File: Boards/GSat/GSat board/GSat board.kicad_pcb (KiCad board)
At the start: 2 copper layers, 75 x 108 mm, 33 parts, among them IC2 MCP23017-E_SP, IC3 SP3485CN-L_TR, J1 B3B-XH-A_LF__SN_, J10 Conn_01x05_Pin, J11 Conn_01x06_Pin, J13 B4B-XH-A_LF__SN_, J14 B4B-XH-A_LF__SN_, J15 B4B-XH-A_LF__SN_, J16 B4B-XH-A_LF__SN_, J3 B3B-XH-A_LF__SN_, J4 B3B-XH-A_LF__SN_, J5 1723163304, U1 TMC2209_SILENTSTEPSTICK, U2 TMC2209_SILENTSTEPSTICK, U3 E28-2G4M27SX, U4 LD1117S33TR_SOT223

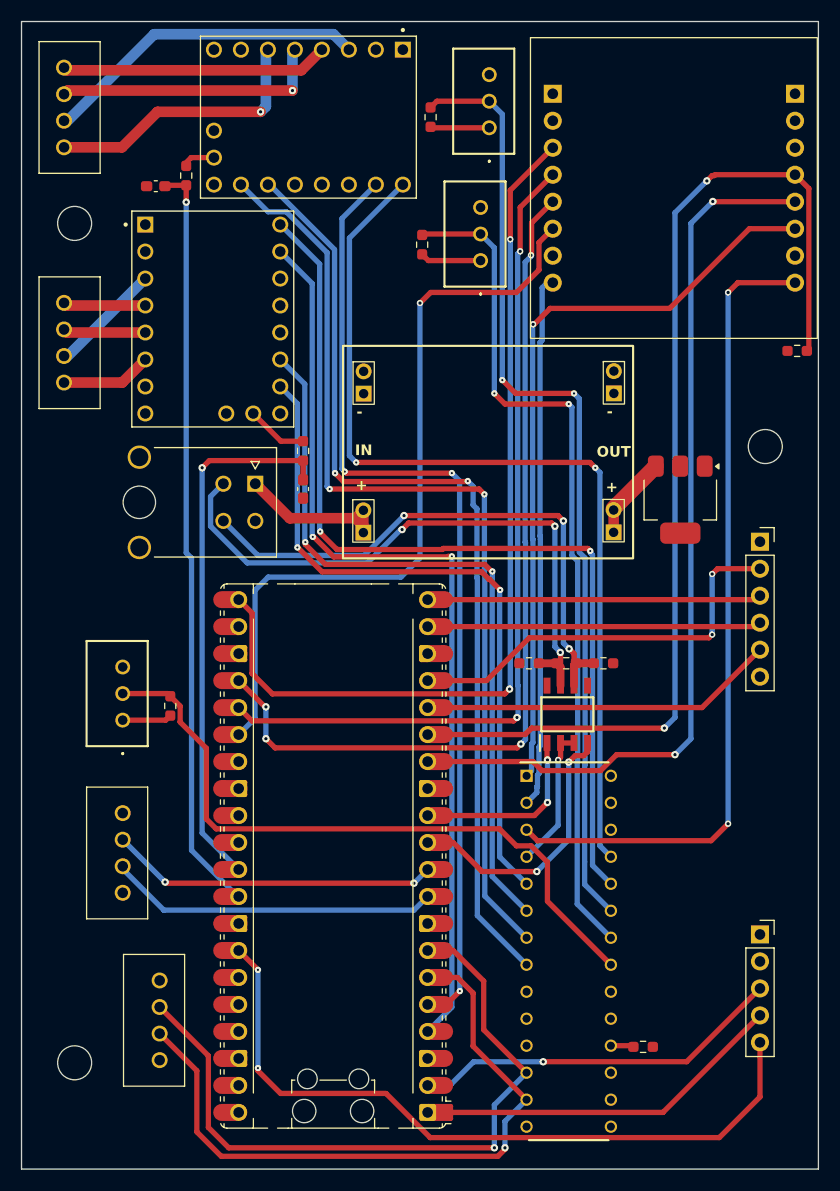
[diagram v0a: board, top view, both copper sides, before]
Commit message: GSPOT update
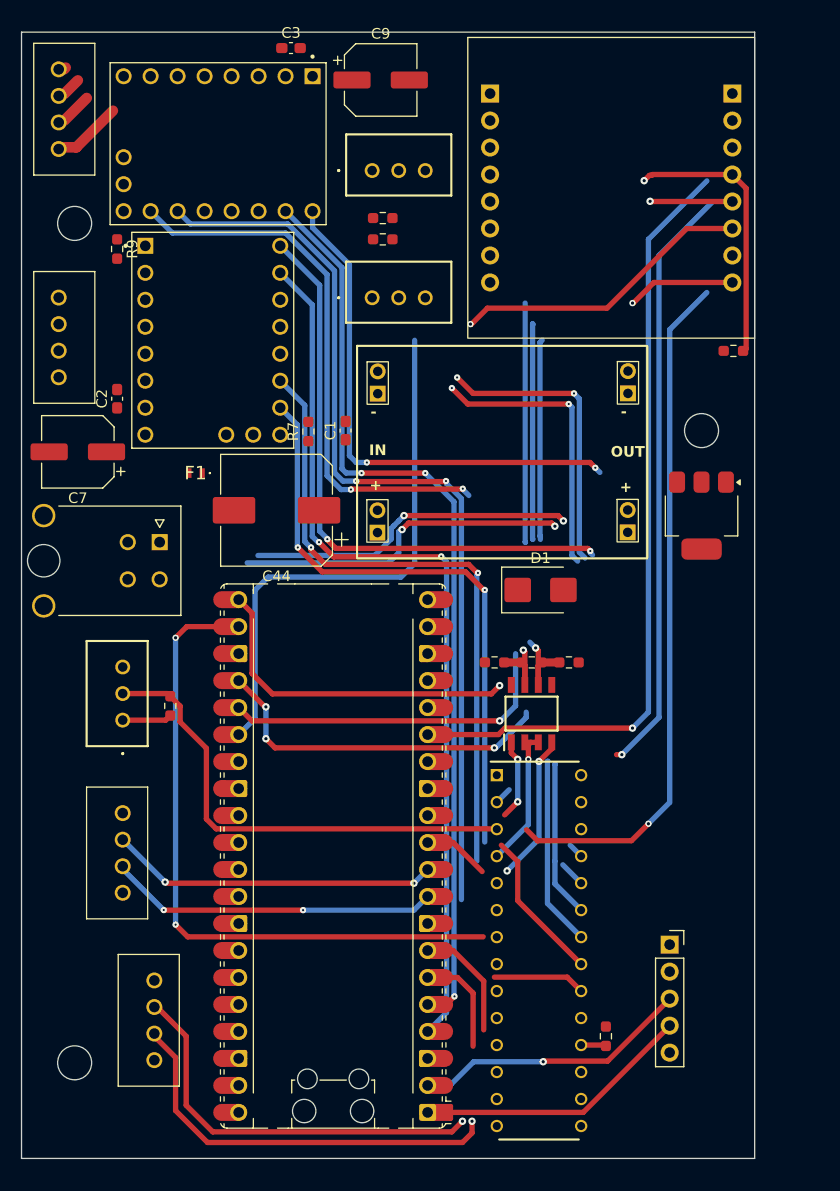
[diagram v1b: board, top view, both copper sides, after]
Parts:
- removed C4, C5: 100n, Capacitor_SMD:C_0603_1608Metric_Pad1.08x0.95mm_HandSolder
- removed J11: Conn_01x06_Pin, Connector_PinSocket_2.54mm:PinSocket_1x06_P2.54mm_Vertical
- removed R6, R8: 1k, Resistor_SMD:R_0603_1608Metric_Pad0.98x0.95mm_HandSolder
- added C1: 100n, Capacitor_SMD:C_0603_1608Metric_Pad1.08x0.95mm_HandSolder, F.Cu at (201.5, 92.5)
- added C2: 100n, Capacitor_SMD:C_0603_1608Metric_Pad1.08x0.95mm_HandSolder, F.Cu at (180.0, 89.5)
- added C3: 100n, Capacitor_SMD:C_0603_1608Metric_Pad1.08x0.95mm_HandSolder, F.Cu at (196.4, 56.5)
- added C44: 470u, Capacitor_SMD:CP_Elec_10x10, F.Cu at (195.0, 100.0)
- added C7: 100u, Capacitor_SMD:CP_Elec_6.3x7.7, F.Cu at (176.3, 94.5)
- added C9: 100u, Capacitor_SMD:CP_Elec_6.3x7.7, F.Cu at (204.8, 59.5)
- added D1: D_Zener, Diode_SMD:D_SMB, F.Cu at (219.8, 107.5)
- added F1: 0ABB-6000-TM, 0ABB-6000-TM:0ABB6000TM, F.Cu at (187.4, 96.5)
- added R7: 10k, Resistor_SMD:R_0603_1608Metric_Pad0.98x0.95mm_HandSolder, F.Cu at (198.0, 92.6)
- added R9: 10k, Resistor_SMD:R_0603_1608Metric_Pad0.98x0.95mm_HandSolder, F.Cu at (180.0, 75.4)
- moved J4 11.7 mm to (204.0, 68.0), turned to 0 degrees
- moved J3 10.8 mm to (204.0, 80.0), turned to 0 degrees
- moved J5 10.5 mm to (184.0, 103.0)
- moved R13 10.5 mm to (205.0, 72.5), turned to 180 degrees
- moved U2 8.86 mm to (189.5, 65.5)
- moved J10 8.55 mm to (232.0, 140.9)
- moved REF** 6.18 mm to (235.0, 92.5)
- moved R2 6.00 mm to (238.0, 85.0)
- moved U3 5.90 mm to (226.5, 69.5)
- moved R12 3.74 mm to (205.0, 74.5), turned to 180 degrees
- moved R14 3.64 mm to (226.0, 149.5), turned to -90 degrees
- moved IC3 3.37 mm to (219.0, 119.1)
- moved R16 3.25 mm to (215.5, 114.3)
- moved R17 3.25 mm to (219.0, 114.3)
- moved R18 3.25 mm to (222.5, 114.3)
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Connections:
- A1 pad 16: /MSD MISO -> /TMC EN
- A1 pad 17: /CS_MSD -> unconnected-(A1-GPIO13-Pad17)
- A1 pad 19: /MSD CLK -> unconnected-(A1-GPIO14-Pad19)
- A1 pad 20: /MSD MOSI -> unconnected-(A1-GPIO15-Pad20)
- A1 pad 31: /Driver1 VREF -> unconnected-(A1-GPIO26_ADC0-Pad31)
- A1 pad 32: /Driver2 VREF -> unconnected-(A1-GPIO27_ADC1-Pad32)
- A1 pad 34: /GPS PPS -> unconnected-(A1-GPIO28_ADC2-Pad34)
- A1 pad 35: GND -> unconnected-(A1-ADC_VREF-Pad35)
- J5 pad 1: +24V -> Net-(F1-Pad2)
- U1 pad 16: +3.3V -> /TMC EN
- U1 pad 18: Net-(U1-DIAG) -> unconnected-(U1-DIAG-Pad18)
- U1 pad 8: +24V -> +12V
- U2 pad 16: +3.3V -> /TMC EN
- U2 pad 18: Net-(U2-DIAG) -> unconnected-(U2-DIAG-Pad18)
- U2 pad 2: +3.3V IC -> +3.3V
- U2 pad 8: +24V -> +12V
- U6 pad 1: +24V -> +12V
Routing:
- net /EXP INTERRUPT: track 0.00 -> 71.5 mm, vias 0 -> 2
- net /Driver2 VREF: track 71.1 -> 0.00 mm, vias 1 -> 0
- net /GPS PPS: track 68.6 -> 0.00 mm, vias 2 -> 0
- net /RADIO MISO: track 85.3 -> 31.9 mm, vias 2 -> 1
- net /Driver1 VREF: track 50.8 -> 0.00 mm, vias 1 -> 0
- net /LimitSwitch3: track 90.0 -> 42.3 mm
- net /RADIO MOSI: track 79.3 -> 32.1 mm, vias 2 -> 1
- net /Driver2 MS1: track 91.3 -> 52.2 mm
- net /Driver2 Dir: track 88.4 -> 50.1 mm
- net /CS_MSD: track 38.2 -> 0.00 mm, vias 2 -> 0
- net /LimitSwitch2: track 80.4 -> 44.6 mm
- net /MSD MISO: track 33.7 -> 0.00 mm
- net /Driver1 Dir: track 88.9 -> 57.6 mm
- net /MSD MOSI: track 30.9 -> 0.00 mm
- net /MSD CLK: track 30.7 -> 0.00 mm
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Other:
- board size 75 x 108 mm -> 69 x 106 mm
